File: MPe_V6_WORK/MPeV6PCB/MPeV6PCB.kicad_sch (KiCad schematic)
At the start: 73 parts, among them J1 UART, J10 TO, J2 SPI, J3 D9, J4 D4, J5 A2, J6 PAS2, J7 TIN, J8 BAT, J9 CUR, SW1 SW_DIP_x02, SW2 SW_DIP_x02, SW3 JP1, U3 Step-down 12V, U4 Step-down 5V

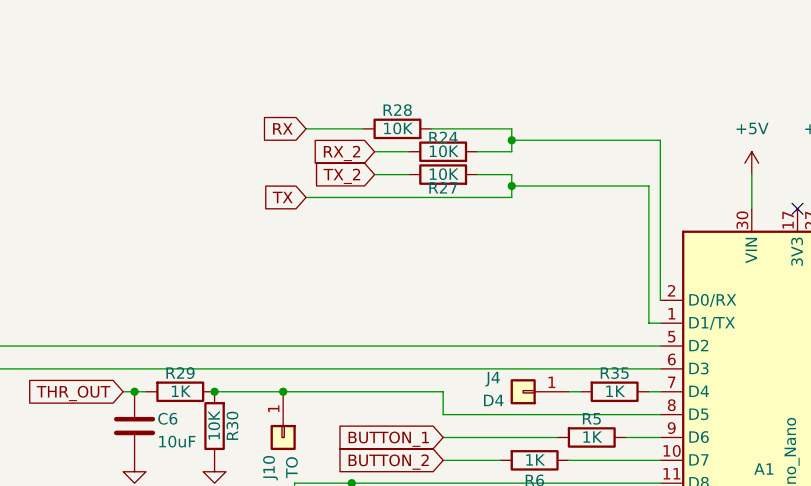
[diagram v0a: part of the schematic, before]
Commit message: zmiana
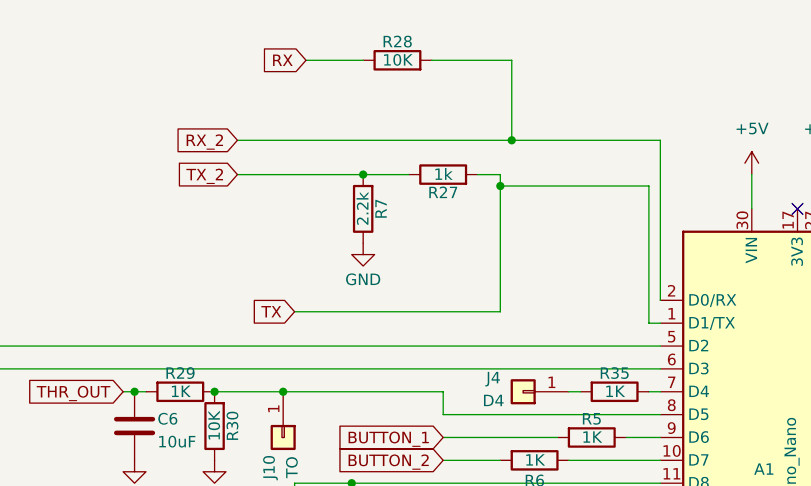
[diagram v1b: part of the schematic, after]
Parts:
- removed R24: 10K, Resistor_SMD:R_0805_2012Metric_Pad1.20x1.40mm_HandSolder, symbol Device:R
- added R7: 2.2k, Resistor_SMD:R_0805_2012Metric_Pad1.20x1.40mm_HandSolder, symbol Device:R
- R27: value 10K -> 1k
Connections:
- net GND: now also R7.1
- net RX_2: now also A1.2 (D0/RX), R28.2
- net TX_2: now also R7.2
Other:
- moved on the sheet: R28
